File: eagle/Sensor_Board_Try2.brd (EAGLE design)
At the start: 69.8 x 64.4 mm, 32 parts, among them IC1 AT24CP, IC3 DS1307, Q1 BSS123, Q2 BSS123, Q3 32.768

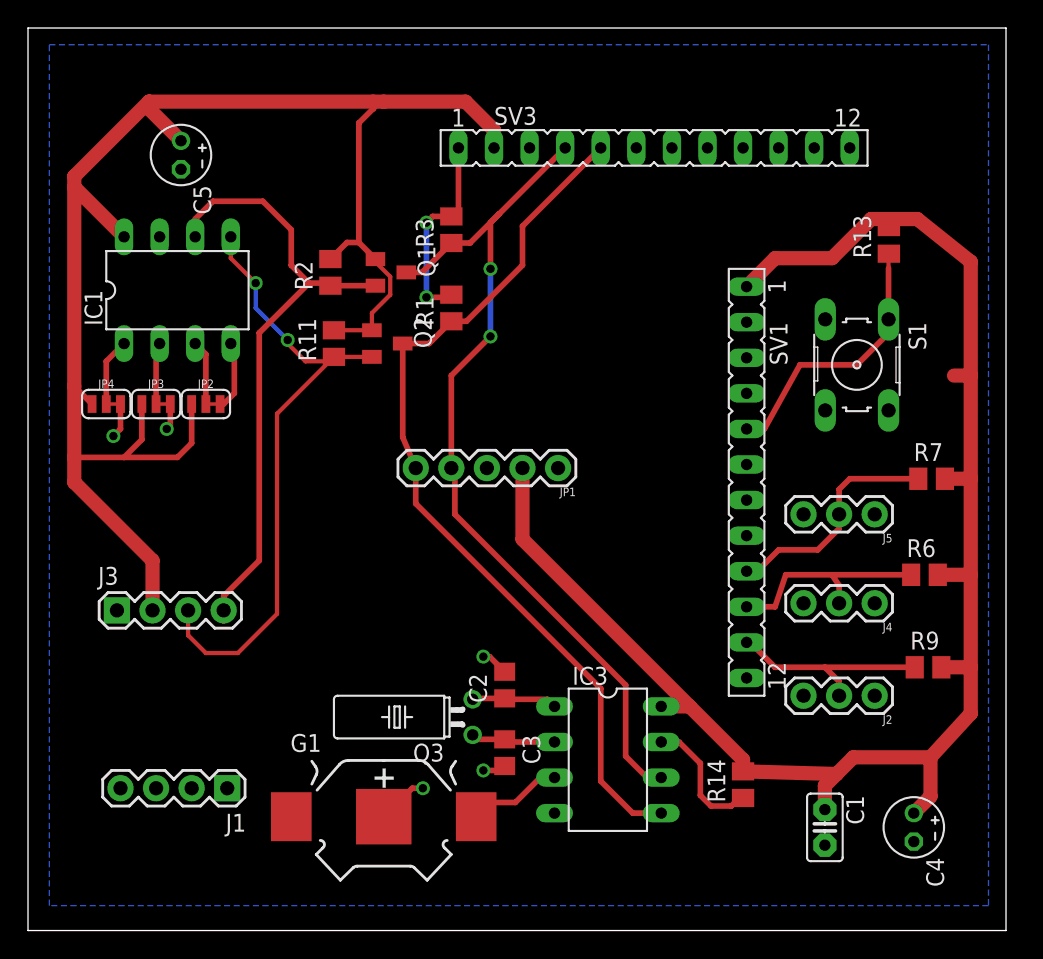
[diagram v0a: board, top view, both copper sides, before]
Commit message: few changes to the board
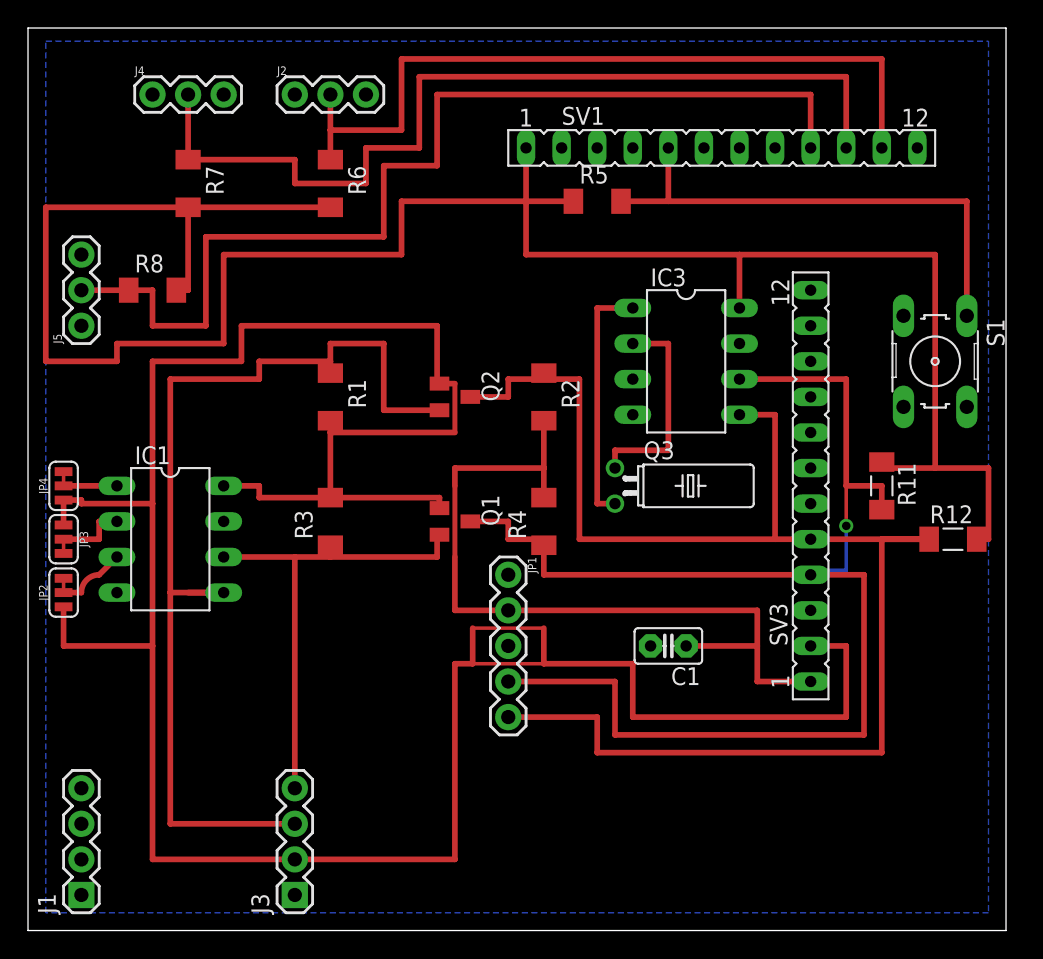
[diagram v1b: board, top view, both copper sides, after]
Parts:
- removed C2, C3: 12.5pF, eagle-ltspice:C0805
- removed C4, C5: (no value), rcl:E2-4
- removed G1: 10MM_SM_COIN_CELL_CLIP, battery:10MM_SM_COIN_CELL_CLIP
- removed R13: 10k, rcl:M0805
- removed R14, R9: 4.7k, rcl:M0805
- added R12: 4.7K, adafruit:M1406
- added R4: 10K, resistor:M1406
- added R5: 10k, rcl:M1406
- added R8: 4.7K, resistor:M1406
- JP2: value JP2 -> JUMPER-SMT_3_1-NC_TRACE_SILK
- JP3: value JP3 -> JUMPER-SMT_3_1-NC_TRACE_SILK
- JP4: value JP4 -> JUMPER-SMT_3_1-NC_TRACE_SILK
- R1, R2, R3: value 10k -> 10K; device rcl:M0805 -> resistor:M1406
- R11: value 10k -> 4.7K; device rcl:M0805 -> adafruit:M1406
- R6, R7: value 4.7k -> 4.7K; device rcl:M0805 -> resistor:M1406
- moved J4 63.1 mm to (16.5, 59.7), turned to 0 degrees
- moved J2 59.6 mm to (26.7, 59.7), turned to 0 degrees
- moved J5 58.2 mm to (11.4, 43.2), turned to 90 degrees
- moved R7 57.1 mm to (19.1, 53.3), turned to 270 degrees
- moved R6 50.8 mm to (29.2, 53.3), turned to 270 degrees
- moved R11 40.4 mm to (68.6, 31.8), turned to 270 degrees
- moved IC3 29.0 mm to (54.6, 40.6)
- moved SV3 26.6 mm to (63.5, 31.8), turned to 90 degrees
- moved J3 24.0 mm to (26.7, 2.54), turned to 90 degrees
- moved SV1 23.9 mm to (57.1, 55.9), turned to 0 degrees
- moved R3 22.5 mm to (29.2, 29.2)
- moved Q3 19.4 mm to (49.5, 31.8), turned to 270 degrees
- moved Q1 18.4 mm to (38.1, 29.2)
- moved IC1 17.8 mm to (17.8, 27.9), turned to 270 degrees
- moved R2 17.6 mm to (44.5, 38.1), turned to 270 degrees
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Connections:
- net 3V: now also R1.2, R3.2; no longer C5.+, R11.2, R2.2
- net 5V: now also R11.1, R12.2, R2.2, R4.2, R5.1, R8.2; no longer C4.+, R1.2, R13.2, R14.2, R3.2, R9.2
- net GND: no longer C2.2, C3.2, C4.-, C5.-, G1.-
- net N$14: no longer C2.1
- net N$15: no longer C3.1
- net N$6: no longer G1.+@1, G1.+@2
- net PD5: now also R6.1; no longer R9.1
- net PD6: now also R7.1; no longer R6.1
- net PD7: now also R8.1; no longer R7.1
- net RESET: now also R5.2; no longer R13.1
- net SCL: now also R11.2, R4.1; no longer R3.1
- net SCLL: now also R3.1; no longer R2.1
- net SDA: now also R12.1, R2.1; no longer R1.1
- net SDAL: now also R1.1; no longer R11.1
- net SQW: no longer R14.1
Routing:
- net 5V: track 128.6 -> 214.6 mm, vias 2 -> 0
- net 3V: track 118.5 -> 201.3 mm
- net PD7: track 16.8 -> 74.9 mm
- net PD6: track 15.6 -> 66.0 mm
- net SDA: track 63.7 -> 105.2 mm
- net PD5: track 15.0 -> 55.4 mm
- net SCL: track 63.5 -> 100.7 mm, vias 2 -> 1
- net SDAL: track 45.8 -> 74.4 mm, vias 2 -> 0
- net RESET: track 19.5 -> 36.7 mm
- net GND: track 16.9 -> 0.00 mm, vias 5 -> 0
- net SCLL: track 46.1 -> 34.4 mm
- net N$14: track 6.11 -> 17.8 mm
- net SQW: track 9.31 -> 0.00 mm
- net N$15: track 6.05 -> 15.2 mm
- net N$6: track 6.75 -> 0.00 mm
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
